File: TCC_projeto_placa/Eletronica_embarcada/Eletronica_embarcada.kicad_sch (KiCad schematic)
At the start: 85 parts, among them J3 BOOT_JUMPER, J4 BUZZER

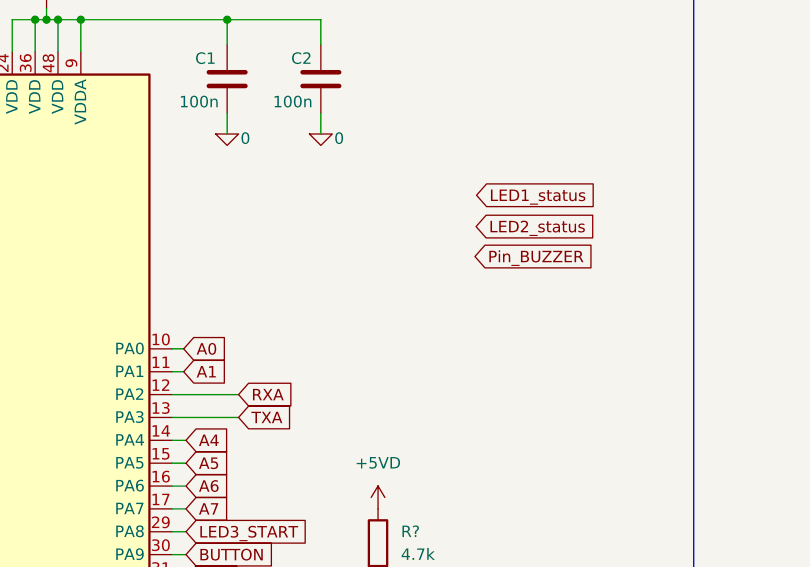
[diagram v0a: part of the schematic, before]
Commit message: att
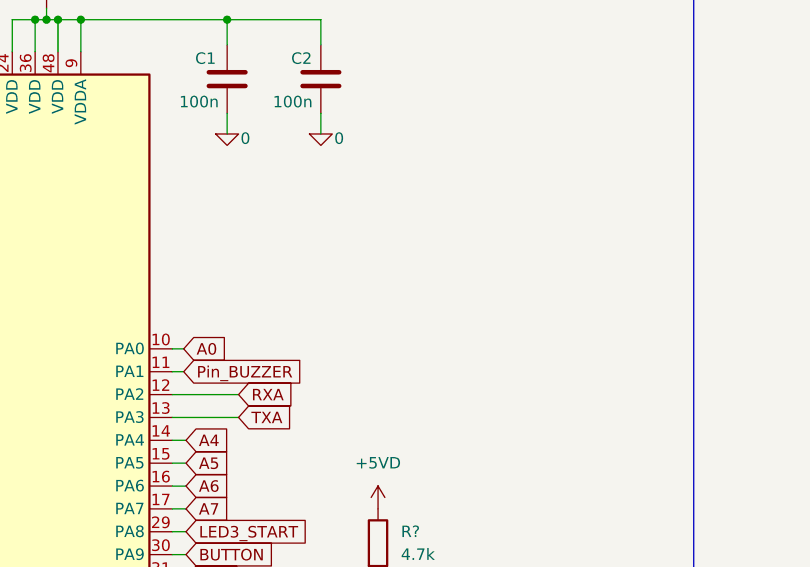
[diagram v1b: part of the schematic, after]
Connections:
- net A1: no longer U?.11 (PA1)
- net Pin_BUZZER: now also U?.11 (PA1)
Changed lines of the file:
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@@
-    )
-  )
-  (global_label "LED2_status" (shape input) (at 305.5366 47.371 0) (fields_autoplaced)
-    (effects (font (size 1.27 1.27)) (justify left))
-    (property "Intersheet References" "${INTERSHEET_REFS}" (id 0) (at 319.3797 47.2916 0)
-      (effects (font (size 1.27 1.27)) (justify left) hide)
     )
   )
@@
     )
   )
-  (global_label "A1" (shape input) (at 273.05 63.5 0) (fields_autoplaced)
-    (effects (font (size 1.27 1.27)) (justify left))
-    (property "Intersheet References" "${INTERSHEET_REFS}" (id 0) (at 277.7612 63.4206 0)
-      (effects (font (size 1.27 1.27)) (justify left) hide)
-    )
-  )
   (global_label "Reset" (shape input) (at 150.5458 43.2054 180) (fields_autoplaced)
     (effects (font (size 1.27 1.27)) (justify right))
@@
     )
   )
-  (global_label "Pin_BUZZER" (shape input) (at 305.4096 50.6984 0) (fields_autoplaced)
-    (effects (font (size 1.27 1.27)) (justify left))
-    (property "Intersheet References" "${INTERSHEET_REFS}" (id 0) (at 319.2527 50.7778 0)
-      (effects (font (size 1.27 1.27)) (justify left) hide)
-    )
-  )
   (global_label "B7" (shape input) (at 382.27 44.45 180) (fields_autoplaced)
     (effects (font (size 1.27 1.27)) (justify right))
@@
     )
   )
-  (global_label "LED1_status" (shape input) (at 305.5874 43.8912 0) (fields_autoplaced)
-    (effects (font (size 1.27 1.27)) (justify left))
-    (property "Intersheet References" "${INTERSHEET_REFS}" (id 0) (at 319.4305 43.8118 0)
-      (effects (font (size 1.27 1.27)) (justify left) hide)
-    )
-  )
   (global_label "BOOT0" (shape input) (at 362.3564 146.5326 180) (fields_autoplaced)
     (effects (font (size 1.27 1.27)) (justify right))
@@
     )
   )
+  (global_label "Pin_BUZZER" (shape input) (at 273.05 63.5 0) (fields_autoplaced)
+    (effects (font (size 1.27 1.27)) (justify left))
+    (property "Intersheet References" "${INTERSHEET_REFS}" (id 0) (at 286.8931 63.5794 0)
+      (effects (font (size 1.27 1.27)) (justify left) hide)
+    )
+  )
